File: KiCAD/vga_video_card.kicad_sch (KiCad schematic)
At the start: 16 parts, among them J1 DE15_Socket_HighDensity, J6 Conn_02x20_Odd_Even, SW1 rst_btn, SW2 SW_DPDT_x2, SW3 SW_DPDT_x2, SW4 SW_DPDT_x2, U27 74HC04, U39 74HC02, Y1 10MHz

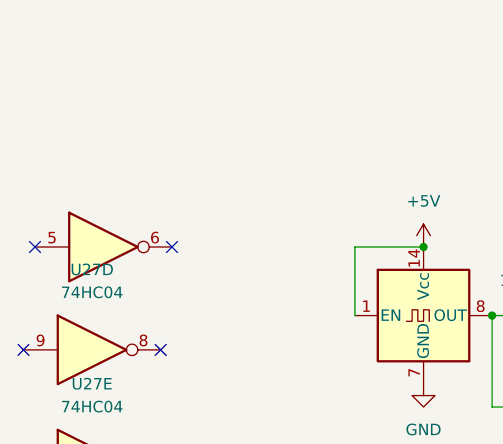
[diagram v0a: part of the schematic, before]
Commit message: update pcb
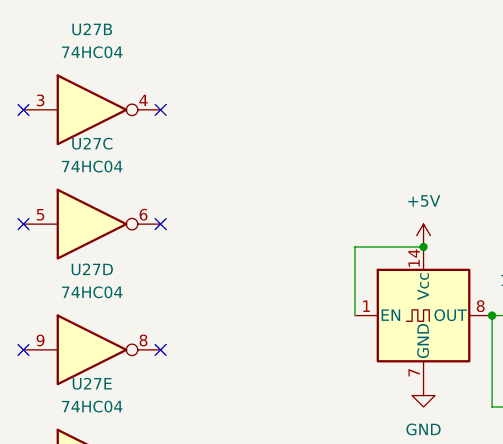
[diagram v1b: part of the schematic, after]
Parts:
- added unit 2 of U27
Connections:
- no-connect marks 14 -> 16
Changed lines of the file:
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@@
 	)
 	(no_connect
-		(at 16.51 34.29)
+		(at 15.24 31.75)
 	)
 	(no_connect
@@
 	)
 	(no_connect
+		(at 30.48 19.05)
+	)
+	(no_connect
 		(at 16.51 114.3)
 	)
 	(no_connect
-		(at 31.75 34.29)
+		(at 15.24 19.05)
+	)
+	(no_connect
+		(at 30.48 31.75)
 	)
 	(no_connect
@@
 	(symbol
 		(lib_id "74xx:74HC04")
-		(at 24.13 34.29 0)
+		(at 22.86 31.75 0)
 		(unit 3)
 		(exclude_from_sim no)
@@
 		(fields_autoplaced yes)
 		(property "Reference" "U27"
-			(at 24.13 25.4 0)
+			(at 22.86 22.86 0)
 			(effects
 				(font
 					(size 1.27 1.27)
 				)
-				(hide yes)
 			)
 		)
 		(property "Value" "74HC04"
-			(at 24.13 27.94 0)
+			(at 22.86 25.4 0)
 			(effects
 				(font
 					(size 1.27 1.27)
 				)
-				(hide yes)
 			)
 		)
 		(property "Footprint" "Package_DIP:DIP-14_W7.62mm"
-			(at 24.13 34.29 0)
+			(at 22.86 31.75 0)
 			(effects
 				(font
@@
 		)
 		(property "Datasheet" "https://assets.nexperia.com/documents/data-sheet/74HC_HCT04.pdf"
-			(at 24.13 34.29 0)
+			(at 22.86 31.75 0)
 			(effects
 				(font
@@
 		)
 		(property "Description" "Hex Inverter"
-			(at 24.13 34.29 0)
+			(at 22.86 31.75 0)
 			(effects
 				(font
@@
 				)
 			)
+		)
+	)
+	(symbol
+		(lib_id "74xx:74HC04")
+		(at 22.86 19.05 0)
+		(unit 2)
+		(exclude_from_sim no)
+		(in_bom yes)
+		(on_board yes)
+		(dnp no)
+		(fields_autoplaced yes)
+		(property "Reference" "U27"
+			(at 22.86 10.16 0)
+			(effects
+				(font
+					(size 1.27 1.27)
+				)
+			)
+		)
+		(property "Value" "74HC04"
+			(at 22.86 12.7 0)
+			(effects
+				(font
+					(size 1.27 1.27)
+				)
+			)
+		)
+		(property "Footprint" "Package_DIP:DIP-14_W7.62mm"
+			(at 22.86 19.05 0)
+			(effects
+				(font
+					(size 1.27 1.27)
+				)
+				(hide yes)
+			)
+		)
+		(property "Datasheet" "https://assets.nexperia.com/documents/data-sheet/74HC_HCT04.pdf"
+			(at 22.86 19.05 0)
+			(effects
+				(font
+					(size 1.27 1.27)
+				)
+				(hide yes)
+			)
+		)
+		(property "Description" "Hex Inverter"
+			(at 22.86 19.05 0)
+			(effects
+				(font
+					(size 1.27 1.27)
+				)
+				(hide yes)
+			)
+		)
+		(pin "14"
+		)
+		(pin "3"
+		)
+		(pin "10"
+		)
+		(pin "1"
+		)
+		(pin "5"
+		)
+		(pin "11"
+		)
+		(pin "12"
+		)
+		(pin "4"
+		)
+		(pin "7"
+		)
+		(pin "9"
+		)
+		(pin "8"
+		)
+		(pin "13"
+		)
+		(pin "2"
+		)
+		(pin "6"
+		)
+		(instances
+			(project "vga_video_card"
+				(path "/53ebbfbe-eaa1-4706-acc1-611a99db7179"
+					(reference "U27")
+					(unit 2)
+				)
+			)
